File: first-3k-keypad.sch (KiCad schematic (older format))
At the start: 24 parts, among them SW1 SW_Push, U1 ATmega32U4-AU, Y1 16MHz

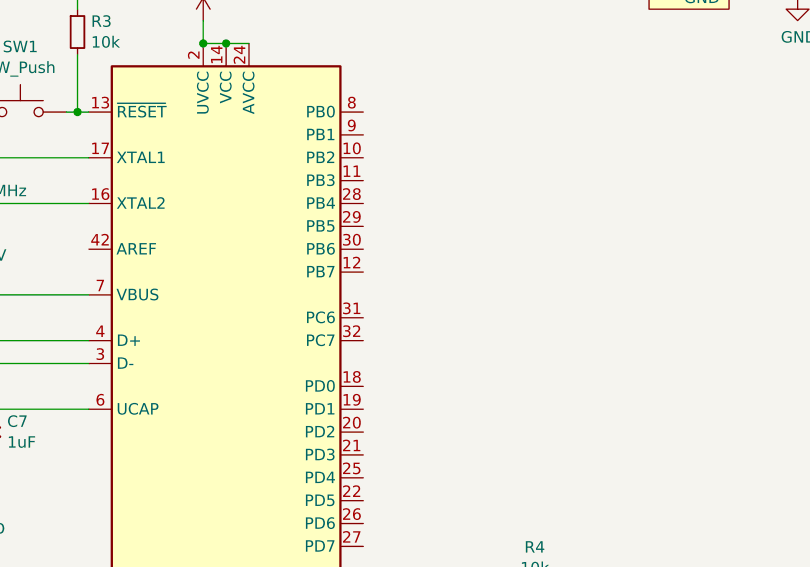
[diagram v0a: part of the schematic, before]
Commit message: Actually Finished this time
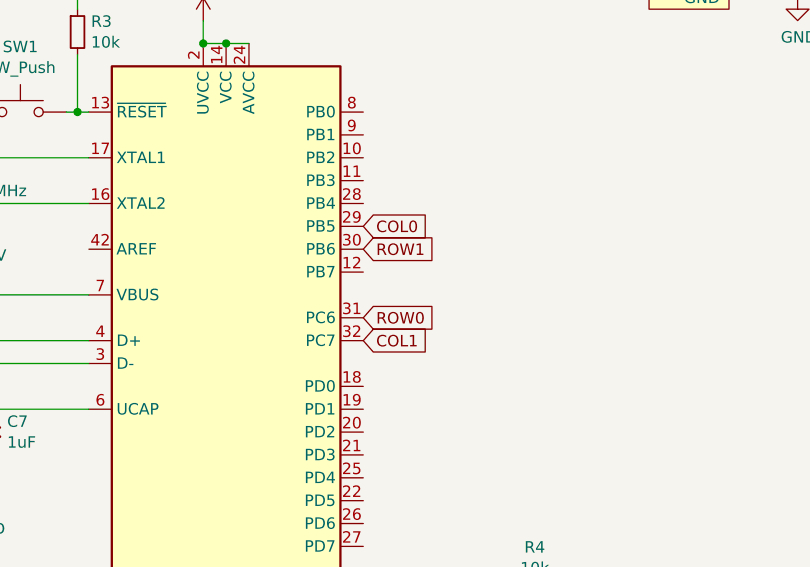
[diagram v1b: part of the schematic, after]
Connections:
- net COL0: now also U1.29 (PB5)
- net COL1: now also U1.31 (PC6), U1.32 (PC7)
- net ROW1: now also U1.30 (PB6)
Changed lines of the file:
@@
 Wire Wire Line
 	10000 3850 10400 3850
+Text GLabel 6400 3400 2    50   Input ~ 0
+COL1
+Text GLabel 6400 2900 2    50   Input ~ 0
+COL0
+Text GLabel 6400 3300 2    50   Input ~ 0
+ROW0
+Text GLabel 6400 3000 2    50   Input ~ 0
+ROW1
 $EndSCHEMATC

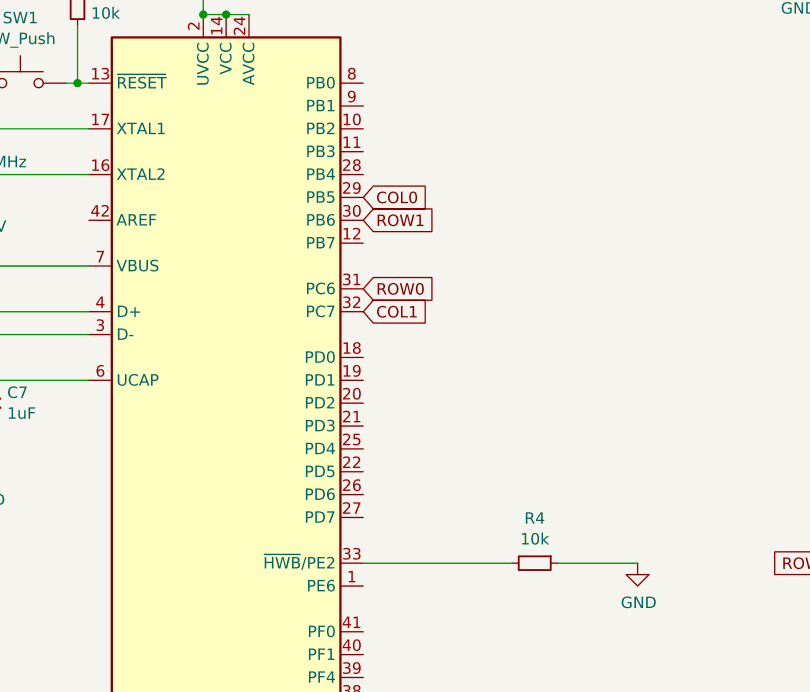
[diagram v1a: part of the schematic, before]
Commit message: New Trace Layout
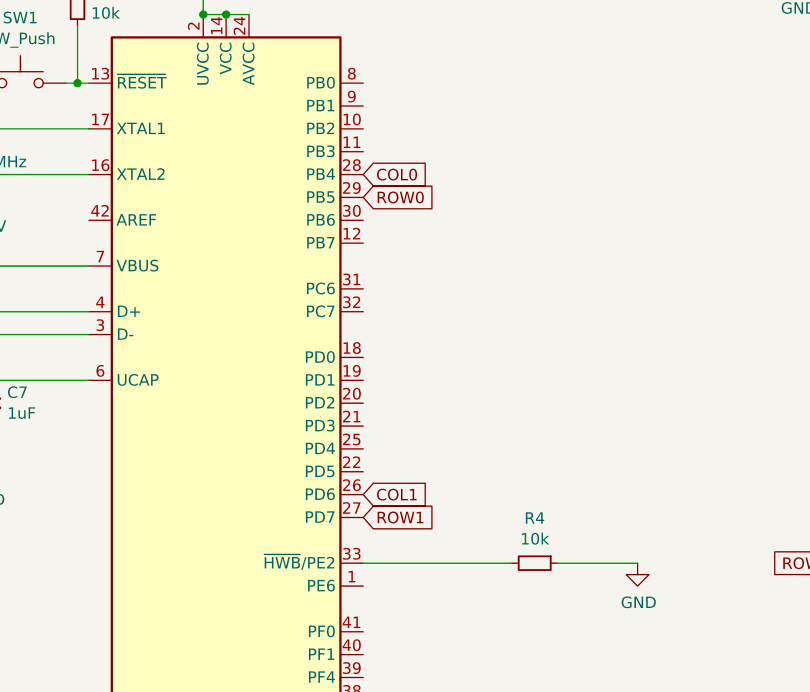
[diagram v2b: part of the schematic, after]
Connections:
- net COL0: now also U1.28 (PB4); no longer U1.29 (PB5)
- net COL1: now also U1.26 (PD6), U1.29 (PB5); no longer U1.31 (PC6), U1.32 (PC7)
- net ROW1: now also U1.27 (PD7); no longer U1.30 (PB6)
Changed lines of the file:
@@
 Wire Wire Line
 	10000 3850 10400 3850
-Text GLabel 6400 3400 2    50   Input ~ 0
+Text GLabel 6400 4200 2    50   Input ~ 0
 COL1
+Text GLabel 6400 2800 2    50   Input ~ 0
+COL0
 Text GLabel 6400 2900 2    50   Input ~ 0
-COL0
-Text GLabel 6400 3300 2    50   Input ~ 0
 ROW0
-Text GLabel 6400 3000 2    50   Input ~ 0
+Text GLabel 6400 4300 2    50   Input ~ 0
 ROW1
 $EndSCHEMATC
